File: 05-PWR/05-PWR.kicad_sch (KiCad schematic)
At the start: 13 parts, among them J1 VDD_IN, J2 GND, J3 VDD_OUT, J4 GND, J5 Ammeter, J6 Voltmeter, J7 Conn_01x04, SW1 SW_DIP_x01, SW2 SW_Push, SW3 SW_SPDT, SW4 SW_Push, SW5 SW_Push

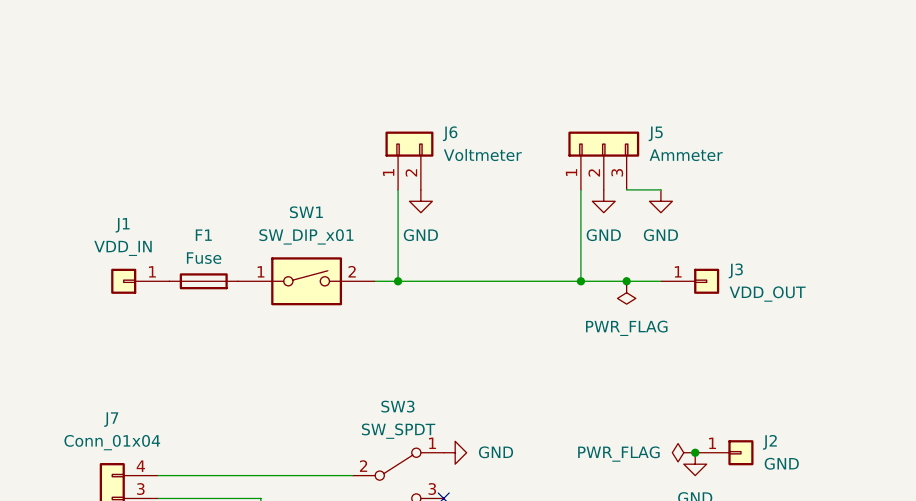
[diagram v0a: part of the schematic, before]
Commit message: 全国行きたかった
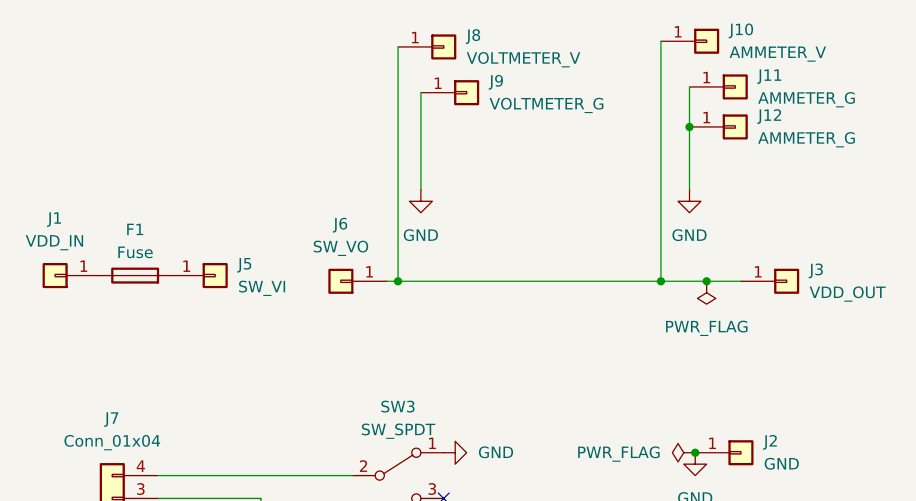
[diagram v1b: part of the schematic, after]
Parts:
- removed J5: Ammeter, Connector_PinSocket_2.54mm:PinSocket_1x03_P2.54mm_Vertical, symbol Connector_Generic:Conn_01x03
- removed J6: Voltmeter, Connector_PinSocket_2.54mm:PinSocket_1x02_P2.54mm_Vertical, symbol Connector_Generic:Conn_01x02
- removed SW1: SW_DIP_x01, Connector_PinHeader_2.54mm:PinHeader_1x02_P2.54mm_Vertical, symbol Switch:SW_DIP_x01
- added J10: AMMETER_V, Connector_PinHeader_2.54mm:PinHeader_1x01_P2.54mm_Vertical, symbol Connector_Generic:Conn_01x01
- added J11, J12: AMMETER_G, Connector_PinHeader_2.54mm:PinHeader_1x01_P2.54mm_Vertical, symbol Connector_Generic:Conn_01x01
- added J5: SW_VI, Connector_PinHeader_2.54mm:PinHeader_1x01_P2.54mm_Vertical, symbol Connector_Generic:Conn_01x01
- added J6: SW_VO, Connector_PinHeader_2.54mm:PinHeader_1x01_P2.54mm_Vertical, symbol Connector_Generic:Conn_01x01
- added J8: VOLTMETER_V, Connector_PinHeader_2.54mm:PinHeader_1x01_P2.54mm_Vertical, symbol Connector_Generic:Conn_01x01
- added J9: VOLTMETER_G, Connector_PinHeader_2.54mm:PinHeader_1x01_P2.54mm_Vertical, symbol Connector_Generic:Conn_01x01
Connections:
- net GND: now also J11.1 (Pin_1), J12.1 (Pin_1), J9.1 (Pin_1)
- net at F1.2: now also J5.1 (Pin_1)
- net at J3.1 (Pin_1): now also J10.1 (Pin_1), J6.1 (Pin_1), J8.1 (Pin_1)
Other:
- moved on the sheet: F1, J1, J3

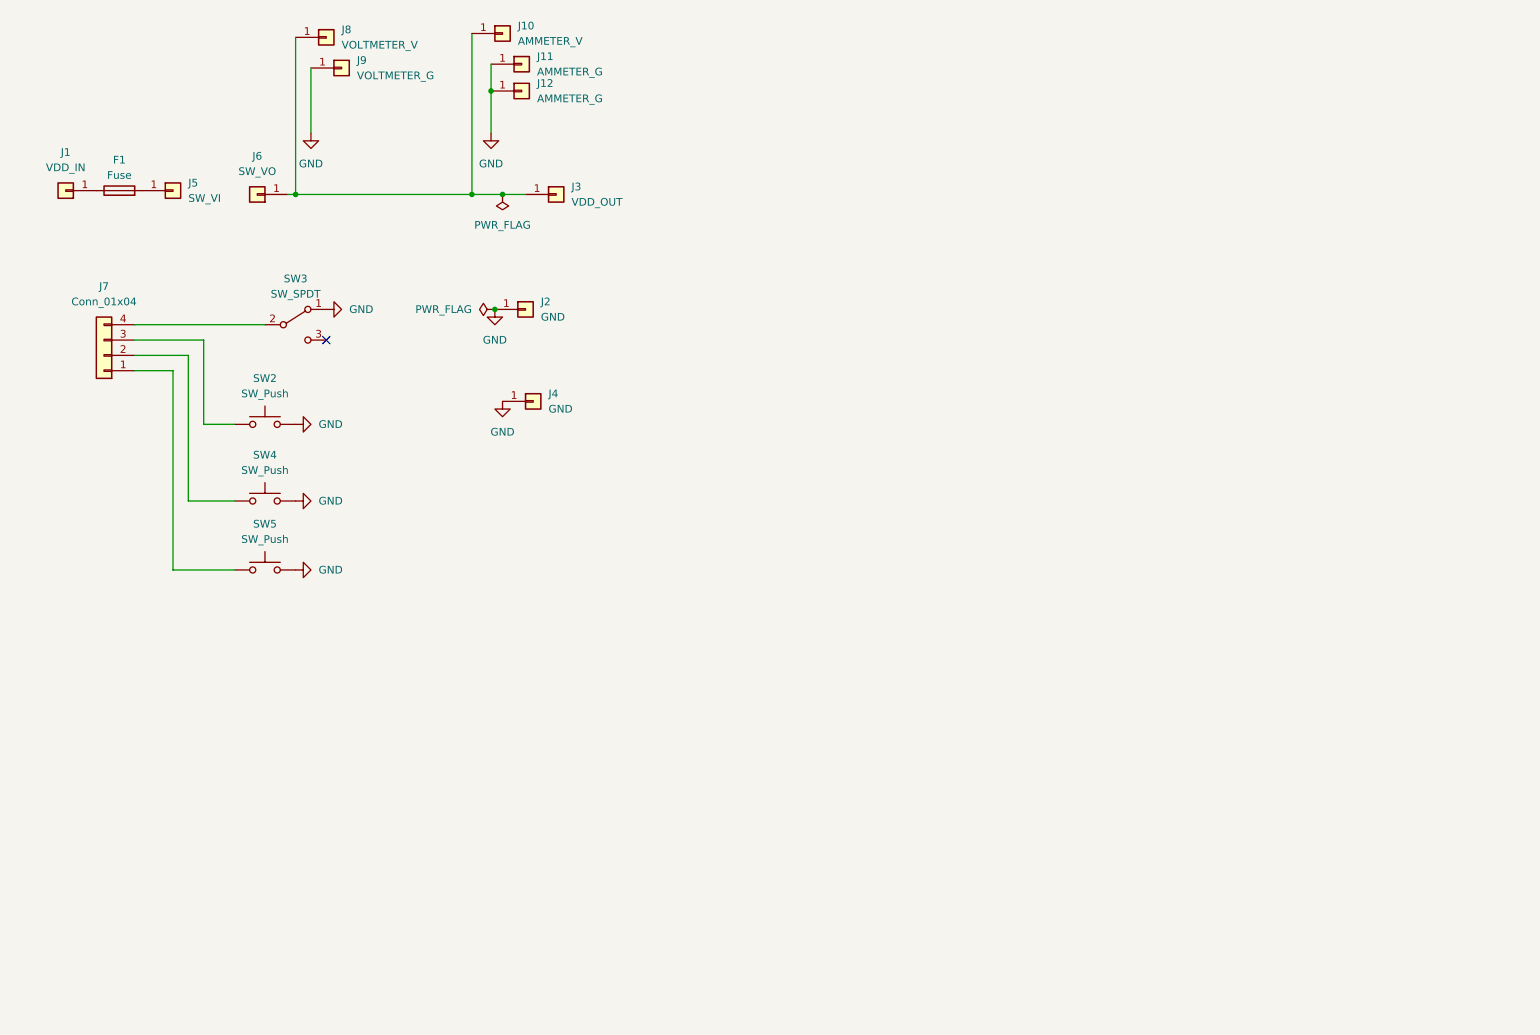
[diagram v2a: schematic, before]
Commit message: いっぱい増えた
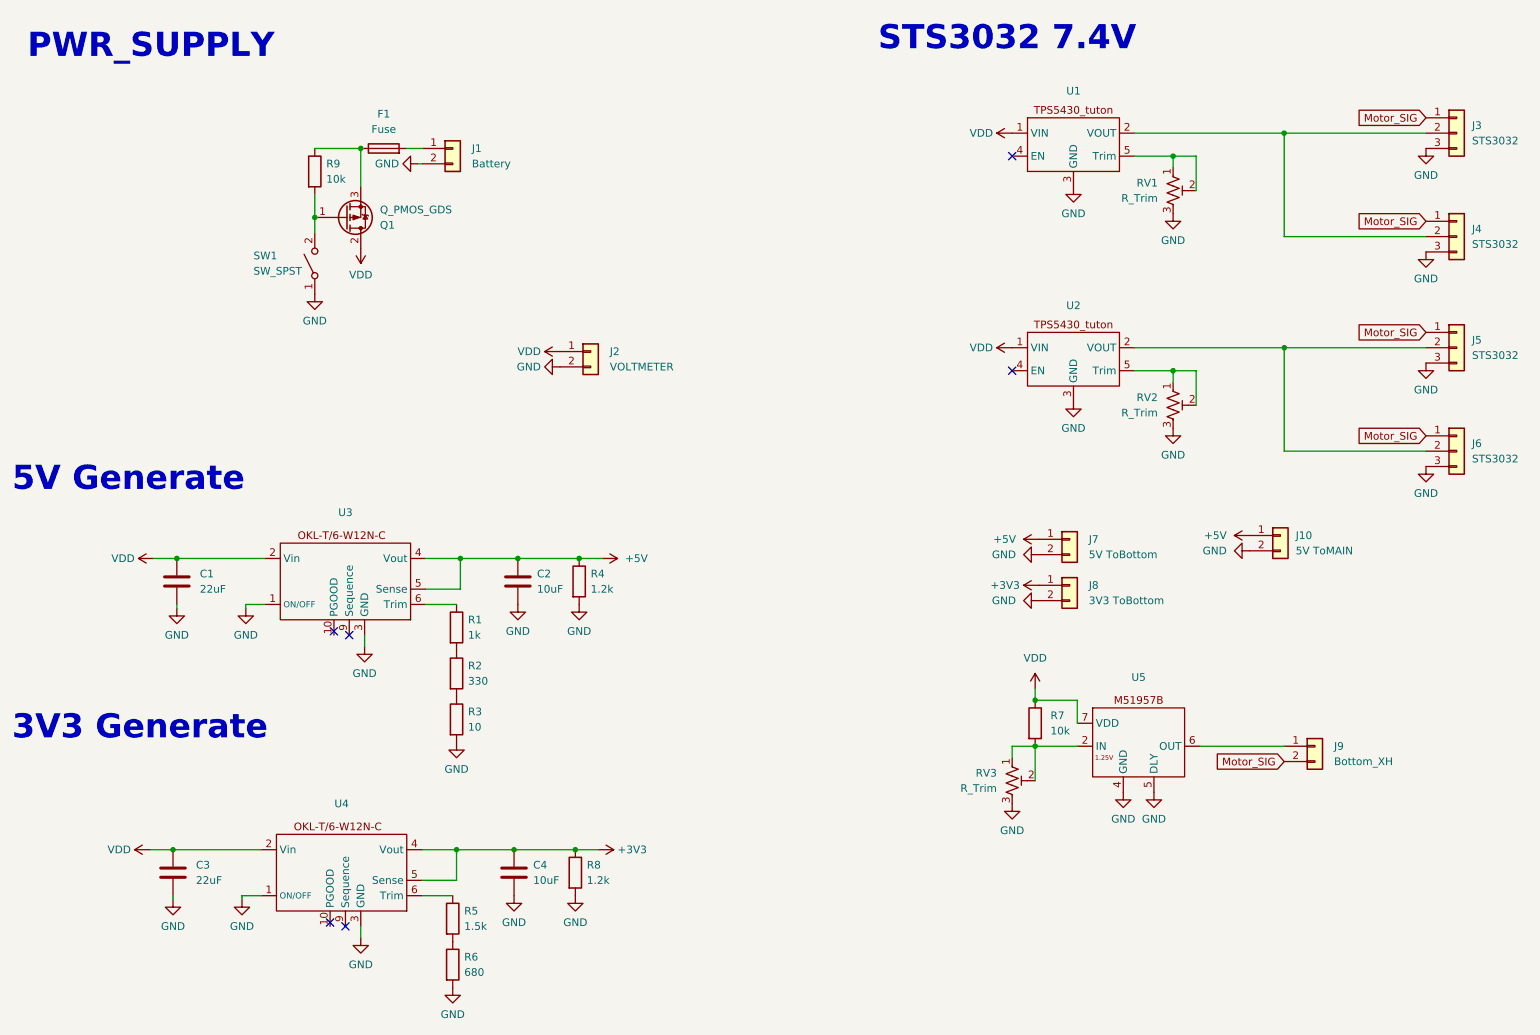
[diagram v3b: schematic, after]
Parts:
- removed J1: VDD_IN, MountingHole:MountingHole_3.2mm_M3_Pad_Via, symbol Connector_Generic:Conn_01x01
- removed J10: AMMETER_V, Connector_PinHeader_2.54mm:PinHeader_1x01_P2.54mm_Vertical, symbol Connector_Generic:Conn_01x01
- removed J11, J12: AMMETER_G, Connector_PinHeader_2.54mm:PinHeader_1x01_P2.54mm_Vertical, symbol Connector_Generic:Conn_01x01
- removed J2, J4: GND, MountingHole:MountingHole_3.2mm_M3_Pad_Via, symbol Connector_Generic:Conn_01x01
- removed J3: VDD_OUT, MountingHole:MountingHole_3.2mm_M3_Pad_Via, symbol Connector_Generic:Conn_01x01
- removed J5: SW_VI, Connector_PinHeader_2.54mm:PinHeader_1x01_P2.54mm_Vertical, symbol Connector_Generic:Conn_01x01
- removed J6: SW_VO, Connector_PinHeader_2.54mm:PinHeader_1x01_P2.54mm_Vertical, symbol Connector_Generic:Conn_01x01
- removed J7: Conn_01x04, Connector_JST:JST_XH_B4B-XH-A_1x04_P2.50mm_Vertical, symbol Connector_Generic:Conn_01x04
- removed J8: VOLTMETER_V, Connector_PinHeader_2.54mm:PinHeader_1x01_P2.54mm_Vertical, symbol Connector_Generic:Conn_01x01
- removed J9: VOLTMETER_G, Connector_PinHeader_2.54mm:PinHeader_1x01_P2.54mm_Vertical, symbol Connector_Generic:Conn_01x01
- removed SW2, SW4, SW5: SW_Push, Button_Switch_THT:SW_PUSH_6mm, symbol Switch:SW_Push
- removed SW3: SW_SPDT, Connector_PinHeader_2.54mm:PinHeader_1x03_P2.54mm_Vertical, symbol Switch:SW_SPDT
- added C1, C3: 22uF, Capacitor_SMD:C_0805_2012Metric, symbol Device:C
- added C2, C4: 10uF, Capacitor_SMD:C_0805_2012Metric, symbol Device:C
- added J1: Battery, Connector_Wire:SolderWire-2sqmm_1x02_P7.8mm_D2mm_OD3.9mm, symbol Connector_Generic:Conn_01x02
- added J10: 5V ToMAIN, Connector_Wire:SolderWire-2sqmm_1x02_P7.8mm_D2mm_OD3.9mm, symbol Connector_Generic:Conn_01x02
- added J2: VOLTMETER, Connector_Wire:SolderWire-2sqmm_1x02_P7.8mm_D2mm_OD3.9mm, symbol Connector_Generic:Conn_01x02
- added J3, J4, J5, J6: STS3032, Connector_JST:JST_XH_B3B-XH-A_1x03_P2.50mm_Vertical, symbol Connector_Generic:Conn_01x03
- added J7: 5V ToBottom, Connector_Wire:SolderWire-2sqmm_1x02_P7.8mm_D2mm_OD3.9mm, symbol Connector_Generic:Conn_01x02
- added J8: 3V3 ToBottom, Connector_Wire:SolderWire-2sqmm_1x02_P7.8mm_D2mm_OD3.9mm, symbol Connector_Generic:Conn_01x02
- added J9: Bottom_XH, Connector_JST:JST_XH_B2B-XH-A_1x02_P2.50mm_Vertical, symbol Connector_Generic:Conn_01x02
- added Q1: Q_PMOS_GDS, Package_TO_SOT_THT:TO-251-3_Vertical, symbol Device:Q_PMOS_GDS
- added R1: 1k, Resistor_SMD:R_0603_1608Metric, symbol Device:R
- added R2: 330, Resistor_SMD:R_0603_1608Metric, symbol Device:R
- added R3: 10, Resistor_SMD:R_0603_1608Metric, symbol Device:R
- added R4, R8: 1.2k, Resistor_SMD:R_0603_1608Metric, symbol Device:R
- added R5: 1.5k, Resistor_SMD:R_0603_1608Metric, symbol Device:R
- added R6: 680, Resistor_SMD:R_0603_1608Metric, symbol Device:R
- added R7, R9: 10k, Resistor_SMD:R_0603_1608Metric, symbol Device:R
- added RV1, RV2, RV3: R_Trim, Potentiometer_THT:Potentiometer_Bourns_3296W_Vertical, symbol Device:R_Potentiometer_Trim_US
- added SW1: SW_SPST, Akiduki:DS-850K-S-ON, symbol Switch:SW_SPST
- added U1, U2: ~, Connector_PinHeader_2.54mm:PinHeader_1x05_P2.54mm_Vertical, symbol tuton_module:TPS5430_module
- added U3, U4: ~, Akiduki:OKL-T6-W12N-C, symbol akiduki:OKL-T/6-W12N-C
- added U5: ~, symbol akiduki:M51957B
- F1: footprint Fuse:Fuseholder_Clip-5x20mm_Keystone_3517_Inline_P23.11x6.76mm_D1.70mm_Horizontal -> (none)
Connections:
- net GND: now also C1.2, C2.2, C3.2, C4.2, J1.2 (Pin_2), J10.2 (Pin_2), J2.2 (Pin_2), J3.3 (Pin_3), J4.3 (Pin_3), J5.3 (Pin_3), J6.3 (Pin_3), J7.2 (Pin_2), J8.2 (Pin_2), R3.2, R4.2, R6.2, R8.2, RV1.3, RV2.3, RV3.3, SW1.1 (A), U1.3 (GND), U2.3 (GND), U3.1 (ON/OFF), U3.3 (GND), U3.7 (GND), U4.1 (ON/OFF), U4.3 (GND), U4.7 (GND), U5.4 (GND), U5.5 (DLY)
- net at F1.1: now also Q1.3 (S), R9.1
- net at F1.2: now also J1.1 (Pin_1)
- new net: Q1.1 (G), R9.2, SW1.2 (B)
- new net: J5.2 (Pin_2), J6.2 (Pin_2), U2.2 (VOUT)
- new net: R2.2, R3.1
- new net: J9.1 (Pin_1), U5.6 (OUT)
- new net: R5.1, U4.6 (Trim)
- new net: R5.2, R6.1
- new net: U5.1 (NC), U5.3 (NC), U5.8 (NC)
- new net: R7.2, RV3.1, RV3.2, U5.2 (IN)
- new net: J3.2 (Pin_2), J4.2 (Pin_2), U1.2 (VOUT)
- new net: R1.1, U3.6 (Trim)
- new net: R1.2, R2.1
- new net: RV2.1, RV2.2, U2.5 (Trim)
- new net: RV1.1, RV1.2, U1.5 (Trim)
- new net +3V3: C4.1, J8.1 (Pin_1), R8.1, U4.4 (Vout), U4.5 (Sense)
- new net +5V: C2.1, J10.1 (Pin_1), J7.1 (Pin_1), R4.1, U3.4 (Vout), U3.5 (Sense)
- new net Motor_SIG: J3.1 (Pin_1), J4.1 (Pin_1), J5.1 (Pin_1), J6.1 (Pin_1), J9.2 (Pin_2)
- new net VDD: C1.1, C3.1, J2.1 (Pin_1), Q1.2 (D), R7.1, U1.1 (VIN), U2.1 (VIN), U3.2 (Vin), U4.2 (Vin), U5.7 (VDD)
- no-connect marks 1 -> 6
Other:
- note added: "3V3 Generate"
- note added: "5V Generate"
- note added: "PWR_SUPPLY"
- note added: "STS3032 7.4V"
